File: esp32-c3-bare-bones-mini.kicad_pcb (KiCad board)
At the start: 4 copper layers, 25.4 x 29.6 mm, 18 parts, among them J3 BATT, U1 ESP32-C3-MINI-1

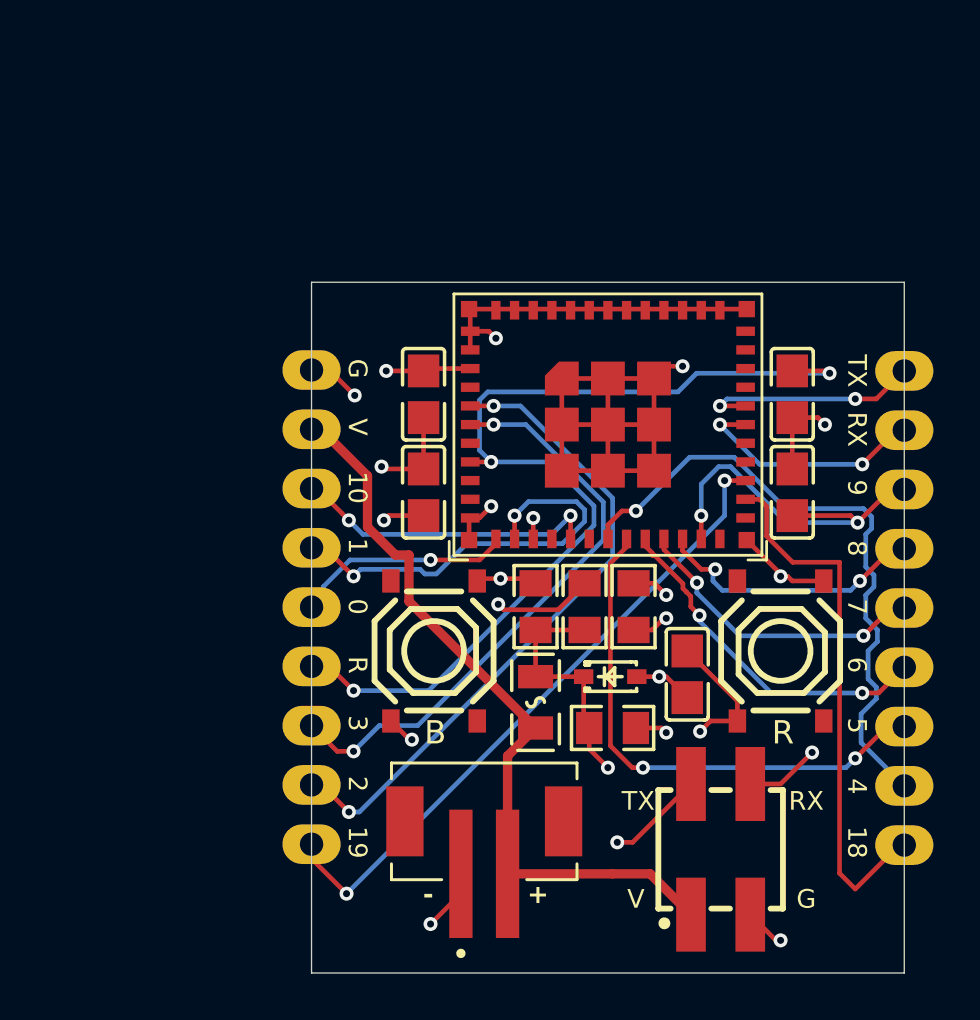
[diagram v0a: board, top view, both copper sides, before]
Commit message: Dual-Mode Power
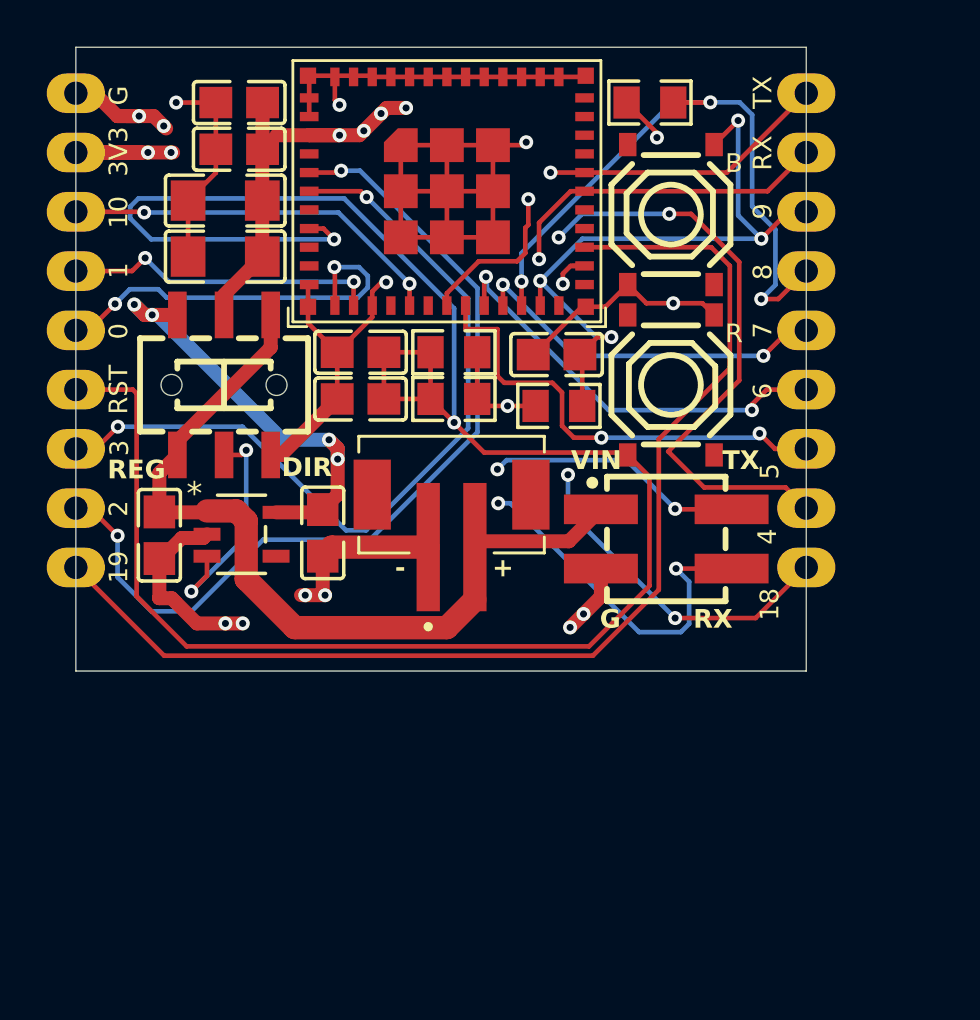
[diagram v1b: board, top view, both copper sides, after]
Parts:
- removed D1: ~, easyeda2kicad:SOD-323_L1.7-W1.3-LS2.6-RD
- removed F1: ~, easyeda2kicad:F0805
- added C6: 1uF 16V 10%, easyeda2kicad:C0805, F.Cu at (124.9, 106.0)
- added C7: 1uF 16V 10%, easyeda2kicad:C0805, F.Cu at (131.9, 105.9)
- added C8: 47uf 10V 20%, CL31A476MPHNNNE:C1206, F.Cu at (127.7, 91.7)
- added C9: 47uf 10V 20%, CL31A476MPHNNNE:C1206, F.Cu at (127.7, 94.1)
- added SW3: Slide Switch, G-Switch MS-22D28-G020:SW-SMD_MS-22D28-G020, F.Cu at (127.7, 99.6)
- added U2: LDO, RT9080-33GJ5:TSOT-23-5_RIT-M, F.Cu at (128.4, 106.0)
- moved R4 26.8 mm to (145.9, 87.5)
- moved B 21.3 mm to (146.8, 92.3)
- moved C1 18.6 mm to (133.5, 98.2), turned to 0 degrees
- moved C5 18.3 mm to (133.5, 100.2), turned to 0 degrees
- moved C3 16.7 mm to (128.3, 89.5), turned to 0 degrees
- moved J1 15.6 mm to (121.3, 97.3)
- moved C2 14.8 mm to (128.3, 87.5), turned to 0 degrees
- moved J3 14.1 mm to (137.4, 104.3)
- moved H1 13.5 mm to (146.6, 106.2), turned to -90 degrees
- moved R1 13.3 mm to (137.5, 98.2), turned to 0 degrees
- moved J2 12.6 mm to (152.6, 97.3)
- moved R 12.3 mm to (146.8, 99.6)
- moved U1 12.1 mm to (137.2, 88.6)
- moved C4 11.7 mm to (141.9, 98.3), turned to 0 degrees
- moved R3 10.5 mm to (137.5, 100.2), turned to 0 degrees
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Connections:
- H1 pad 1: FUSE_VCC -> VCC_IN
- J1 pad 2: FUSE_VCC -> VCC_3V3
- J3 pad 2: FUSE_VCC -> VCC_IN
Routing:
- net VCC_IN: track 0.00 -> 38.2 mm
- net FUSE_VCC: track 32.0 -> 0.00 mm
- net GND: track 65.5 -> 96.5 mm, vias 12 -> 13
- net GPIO19: track 28.1 -> 49.4 mm, vias 2 -> 0
- net Net-(U2-VOUT): track 0.00 -> 19.3 mm, vias 0 -> 4
- net U0RXD: track 26.8 -> 42.9 mm
- net CHIP_PU: track 75.8 -> 90.5 mm, vias 6 -> 2
- net VCC_3V3: track 17.6 -> 31.7 mm, vias 4 -> 8
- net U0TXD: track 35.1 -> 47.5 mm
- net GPIO2: track 28.3 -> 38.8 mm
- net LDO_EN: track 0.00 -> 9.91 mm, vias 0 -> 2
- net GPIO3: track 25.4 -> 35.1 mm
- net GPIO0: track 9.96 -> 17.3 mm, vias 1 -> 2
- net GPIO4: track 28.3 -> 34.5 mm, vias 1 -> 3
- net GPIO1: track 18.2 -> 13.6 mm
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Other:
- board size 25.4 x 29.6 mm -> 31.3 x 26.7 mm
- board text added: "3V3"
- board text added: "DIR"
- board text added: "REG"
- board text added: "RST"
- board text added: "VIN"
- board text added: "bj-dehaan-solutions.com.au"
- board text removed: "R"
- board text removed: "V"
